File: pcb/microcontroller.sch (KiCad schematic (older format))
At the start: 6 parts

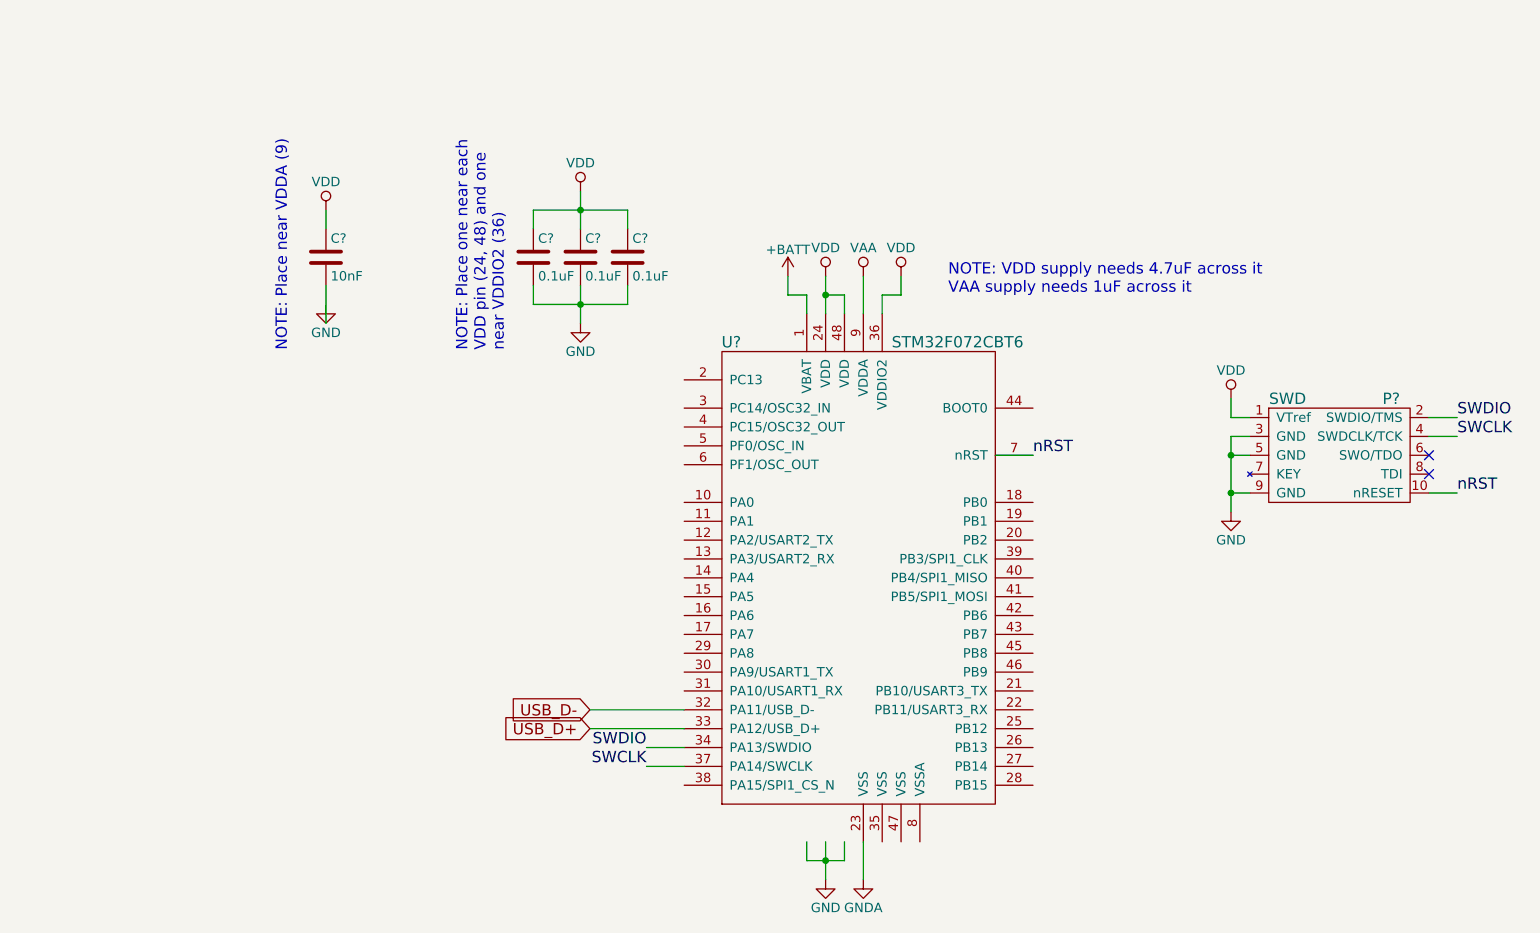
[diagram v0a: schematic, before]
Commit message: Add JSTA-4 connector
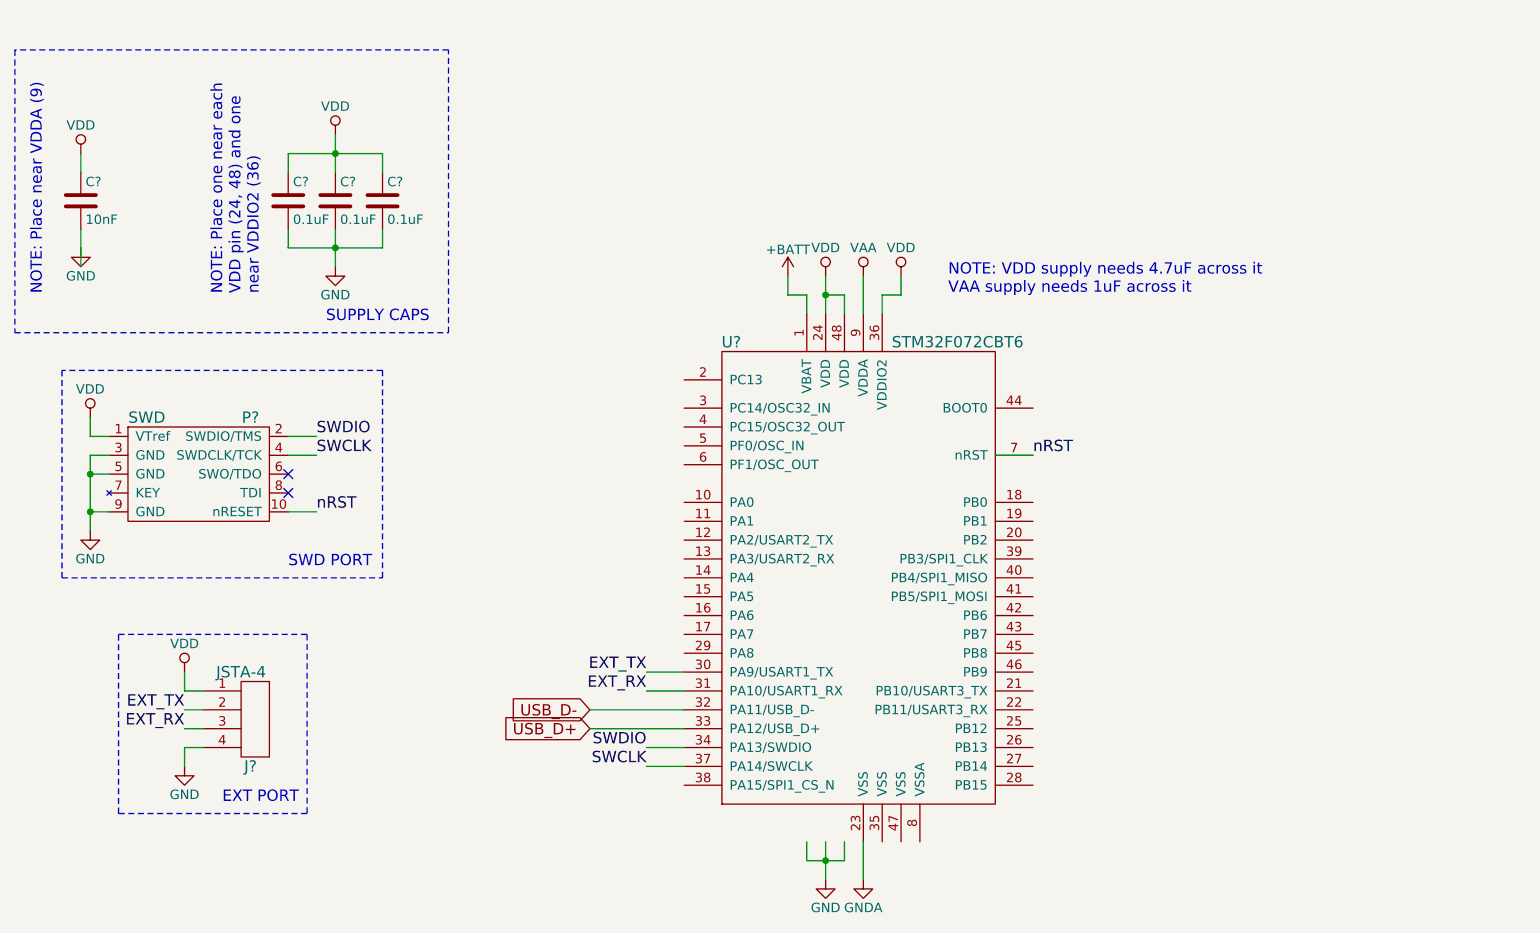
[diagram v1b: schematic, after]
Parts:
- added J?: JSTA-4, symbol JSTA-4
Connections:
- net labels added: EXT_RX, EXT_TX
- wire segments 48 -> 56
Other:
- note added: "EXT PORT"
- note added: "SUPPLY CAPS"
- note added: "SWD PORT"
- moved on the sheet: C?, P?
